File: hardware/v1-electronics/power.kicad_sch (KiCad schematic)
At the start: 44 parts, among them IC1 TPS61288LRQQR, IC2 MP2721GRH-0000-Z, J1 Female USB-C USB2.0, J2 XT30PW-M, Q1 AON7423, SW7 2TED3M6RES

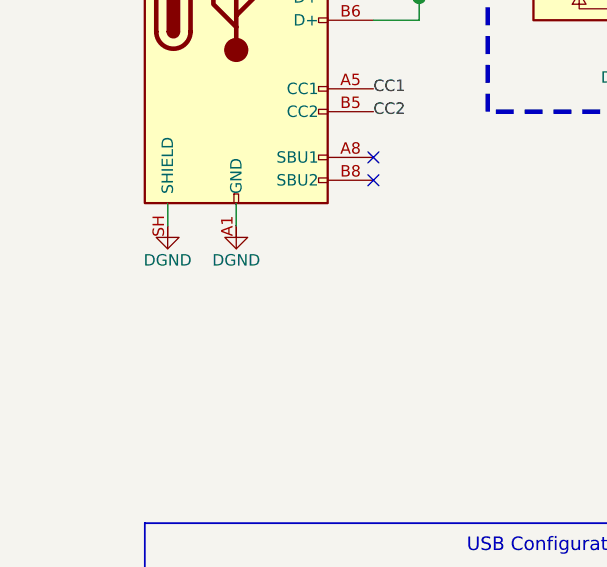
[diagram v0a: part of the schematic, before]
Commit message: feat(v1 hardware): update config switch
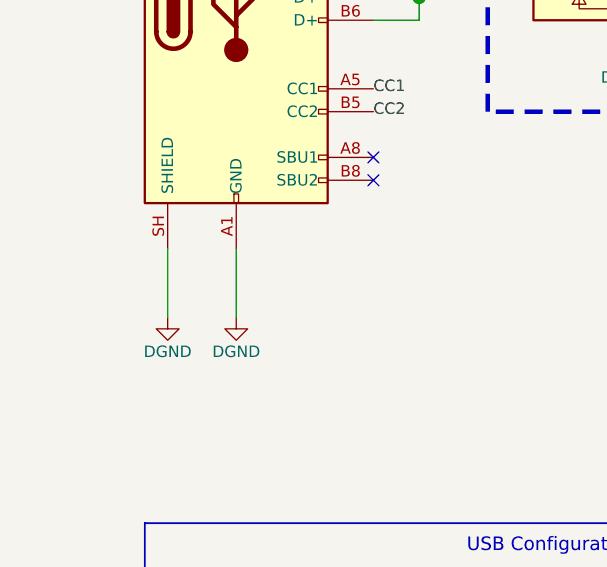
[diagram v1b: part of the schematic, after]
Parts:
- JP5, JP6: footprint Connector_PinHeader_2.54mm:PinHeader_1x02_P2.54mm_Vertical -> Dongguan Guangzhu Industrial:DSIC01LSGET
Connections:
- net DGND: now also J1.A1 (GND), J1.A12 (GND), J1.B1 (GND), J1.B12 (GND), J1.SH (SHIELD)
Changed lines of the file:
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@@
 	)
 	(junction
-		(at 55.88 111.76)
-		(diameter 1.5)
-		(color 0 0 255 1)
-	)
-	(junction
 		(at 302.26 101.6)
 		(diameter 1.5)
@@
 	)
 	(junction
+		(at 55.88 111.76)
+		(diameter 1.5)
+		(color 0 0 255 1)
+	)
+	(junction
 		(at 160.02 104.14)
 		(diameter 1.5)
@@
 	)
 	(junction
-		(at 182.88 96.52)
+		(at 55.88 106.68)
 		(diameter 1.5)
-		(color 0 0 0 0)
+		(color 0 0 255 1)
 	)
 	(junction
-		(at 309.88 101.6)
+		(at 182.88 96.52)
 		(diameter 1.5)
 		(color 0 0 0 0)
 	)
 	(junction
-		(at 55.88 106.68)
+		(at 309.88 101.6)
 		(diameter 1.5)
-		(color 0 0 255 1)
+		(color 0 0 0 0)
 	)
 	(junction
@@
 	(wire
 		(pts
+			(xy 96.52 198.12) (xy 93.98 195.58)
+		)
+		(stroke
+			(width 0)
+			(type default)
+		)
+	)
+	(wire
+		(pts
 			(xy 55.88 106.68) (xy 55.88 109.22)
 		)
@@
 	(wire
 		(pts
-			(xy 96.52 198.12) (xy 93.98 195.58)
+			(xy 332.74 111.76) (xy 340.36 111.76)
 		)
 		(stroke
-			(width 0)
+			(width 0.5)
 			(type default)
 		)
@@
 	(wire
 		(pts
-			(xy 332.74 111.76) (xy 340.36 111.76)
+			(xy 55.88 111.76) (xy 55.88 114.3)
 		)
 		(stroke
 			(width 0.5)
 			(type default)
+			(color 0 0 255 1)
 		)
 	)
@@
 	(wire
 		(pts
+			(xy 55.88 111.76) (xy 66.04 111.76)
+		)
+		(stroke
+			(width 0.5)
+			(type default)
+			(color 0 0 255 1)
+		)
+	)
+	(wire
+		(pts
 			(xy 302.26 226.06) (xy 304.8 226.06)
 		)
@@
 	(wire
 		(pts
-			(xy 55.88 111.76) (xy 66.04 111.76)
-		)
-		(stroke
-			(width 0.5)
-			(type default)
-			(color 0 0 255 1)
-		)
-	)
-	(wire
-		(pts
 			(xy 414.02 119.38) (xy 414.02 116.84)
 		)
@@
 	(wire
 		(pts
-			(xy 55.88 106.68) (xy 66.04 106.68)
+			(xy 304.8 226.06) (xy 320.04 226.06)
 		)
 		(stroke
-			(width 0.5)
+			(width 0)
 			(type default)
-			(color 0 0 255 1)
 		)
 	)
 	(wire
 		(pts
-			(xy 304.8 226.06) (xy 320.04 226.06)
+			(xy 439.42 88.9) (xy 452.12 88.9)
 		)
 		(stroke
-			(width 0)
+			(width 0.5)
 			(type default)
 		)
@@
 	(wire
 		(pts
-			(xy 439.42 88.9) (xy 452.12 88.9)
+			(xy 302.26 101.6) (xy 302.26 104.14)
 		)
 		(stroke
@@
 	(wire
 		(pts
-			(xy 302.26 101.6) (xy 302.26 104.14)
+			(xy 332.74 147.32) (xy 335.28 147.32)
 		)
 		(stroke
@@
 	(wire
 		(pts
-			(xy 332.74 147.32) (xy 335.28 147.32)
+			(xy 27.94 139.7) (xy 27.94 147.32)
 		)
 		(stroke
-			(width 0.5)
+			(width 0)
 			(type default)
 		)
@@
 	(wire
 		(pts
-			(xy 27.94 137.16) (xy 27.94 134.62)
-		)
-		(stroke
-			(width 0)
-			(type default)
-		)
-	)
-	(wire
-		(pts
 			(xy 149.86 175.26) (xy 165.1 175.26)
 		)
@@
 	(wire
 		(pts
-			(xy 35.56 137.16) (xy 35.56 134.62)
-		)
-		(stroke
-			(width 0)
-			(type default)
-		)
-	)
-	(wire
-		(pts
 			(xy 241.3 182.88) (xy 241.3 180.34)
 		)
@@
 	(wire
 		(pts
-			(xy 55.88 111.76) (xy 55.88 114.3)
-		)
-		(stroke
-			(width 0.5)
-			(type default)
-			(color 0 0 255 1)
-		)
-	)
-	(wire
-		(pts
 			(xy 477.52 91.44) (xy 477.52 88.9)
 		)
@@
 	(wire
 		(pts
+			(xy 55.88 106.68) (xy 66.04 106.68)
+		)
+		(stroke
+			(width 0.5)
+			(type default)
+			(color 0 0 255 1)
+		)
+	)
+	(wire
+		(pts
 			(xy 78.74 96.52) (xy 78.74 101.6)
 		)
@@
 	(wire
 		(pts
+			(xy 35.56 139.7) (xy 35.56 147.32)
+		)
+		(stroke
+			(width 0)
+			(type default)
+		)
+	)
+	(wire
+		(pts
 			(xy 320.04 223.52) (xy 320.04 226.06)
 		)
@@
 			)
 		)
-		(property "Footprint" "Connector_PinHeader_2.54mm:PinHeader_1x02_P2.54mm_Vertical"
+		(property "Footprint" "Dongguan Guangzhu Industrial:DSIC01LSGET"
 			(at 81.28 187.96 0)
 			(hide yes)
@@
 	(symbol
 		(lib_id "power:GND")
-		(at 35.56 137.16 0)
+		(at 35.56 147.32 0)
 		(unit 1)
 		(body_style 1)
@@
 		(dnp no)
 		(property "Reference" "#PWR0104"
-			(at 35.56 143.51 0)
+			(at 35.56 153.67 0)
 			(hide yes)
 			(show_name no)
@@
 		)
 		(property "Value" "DGND"
-			(at 35.5599 140.97 0)
+			(at 35.5599 151.13 0)
 			(show_name no)
 			(do_not_autoplace no)
@@
 		)
 		(property "Footprint" ""
-			(at 35.56 137.16 0)
+			(at 35.56 147.32 0)
 			(hide yes)
 			(show_name no)
@@
 		)
 		(property "Datasheet" ""
-			(at 35.56 137.16 0)
+			(at 35.56 147.32 0)
 			(hide yes)
 			(show_name no)
@@
 		)
 		(property "Description" "Power symbol creates a global label with name \"GND\" , ground"
-			(at 35.56 137.16 0)
+			(at 35.56 147.32 0)
 			(hide yes)
 			(show_name no)
@@
 			)
 		)
-		(property "Footprint" "Connector_PinHeader_2.54mm:PinHeader_1x02_P2.54mm_Vertical"
+		(property "Footprint" "Dongguan Guangzhu Industrial:DSIC01LSGET"
 			(at 99.06 198.12 0)
 			(hide yes)
@@
 	(symbol
 		(lib_id "power:GND")
-		(at 27.94 137.16 0)
+		(at 27.94 147.32 0)
 		(unit 1)
 		(body_style 1)
@@
 		(dnp no)
 		(property "Reference" "#PWR0103"
-			(at 27.94 143.51 0)
+			(at 27.94 153.67 0)
 			(hide yes)
 			(show_name no)
@@
 		)
 		(property "Value" "DGND"
-			(at 27.9399 140.97 0)
+			(at 27.9399 151.13 0)
 			(show_name no)
 			(do_not_autoplace no)
@@
 		)
 		(property "Footprint" ""
-			(at 27.94 137.16 0)
+			(at 27.94 147.32 0)
 			(hide yes)
 			(show_name no)
@@
 		)
 		(property "Datasheet" ""
-			(at 27.94 137.16 0)
+			(at 27.94 147.32 0)
 			(hide yes)
 			(show_name no)
@@
 		)
 		(property "Description" "Power symbol creates a global label with name \"GND\" , ground"
-			(at 27.94 137.16 0)
+			(at 27.94 147.32 0)
 			(hide yes)
 			(show_name no)
